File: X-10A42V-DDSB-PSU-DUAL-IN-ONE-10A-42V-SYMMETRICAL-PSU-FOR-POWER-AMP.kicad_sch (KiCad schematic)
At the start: 61 parts, among them K101 SLA-24VDC-SL-A, SW101 JWMW21RA1A, T101 15A

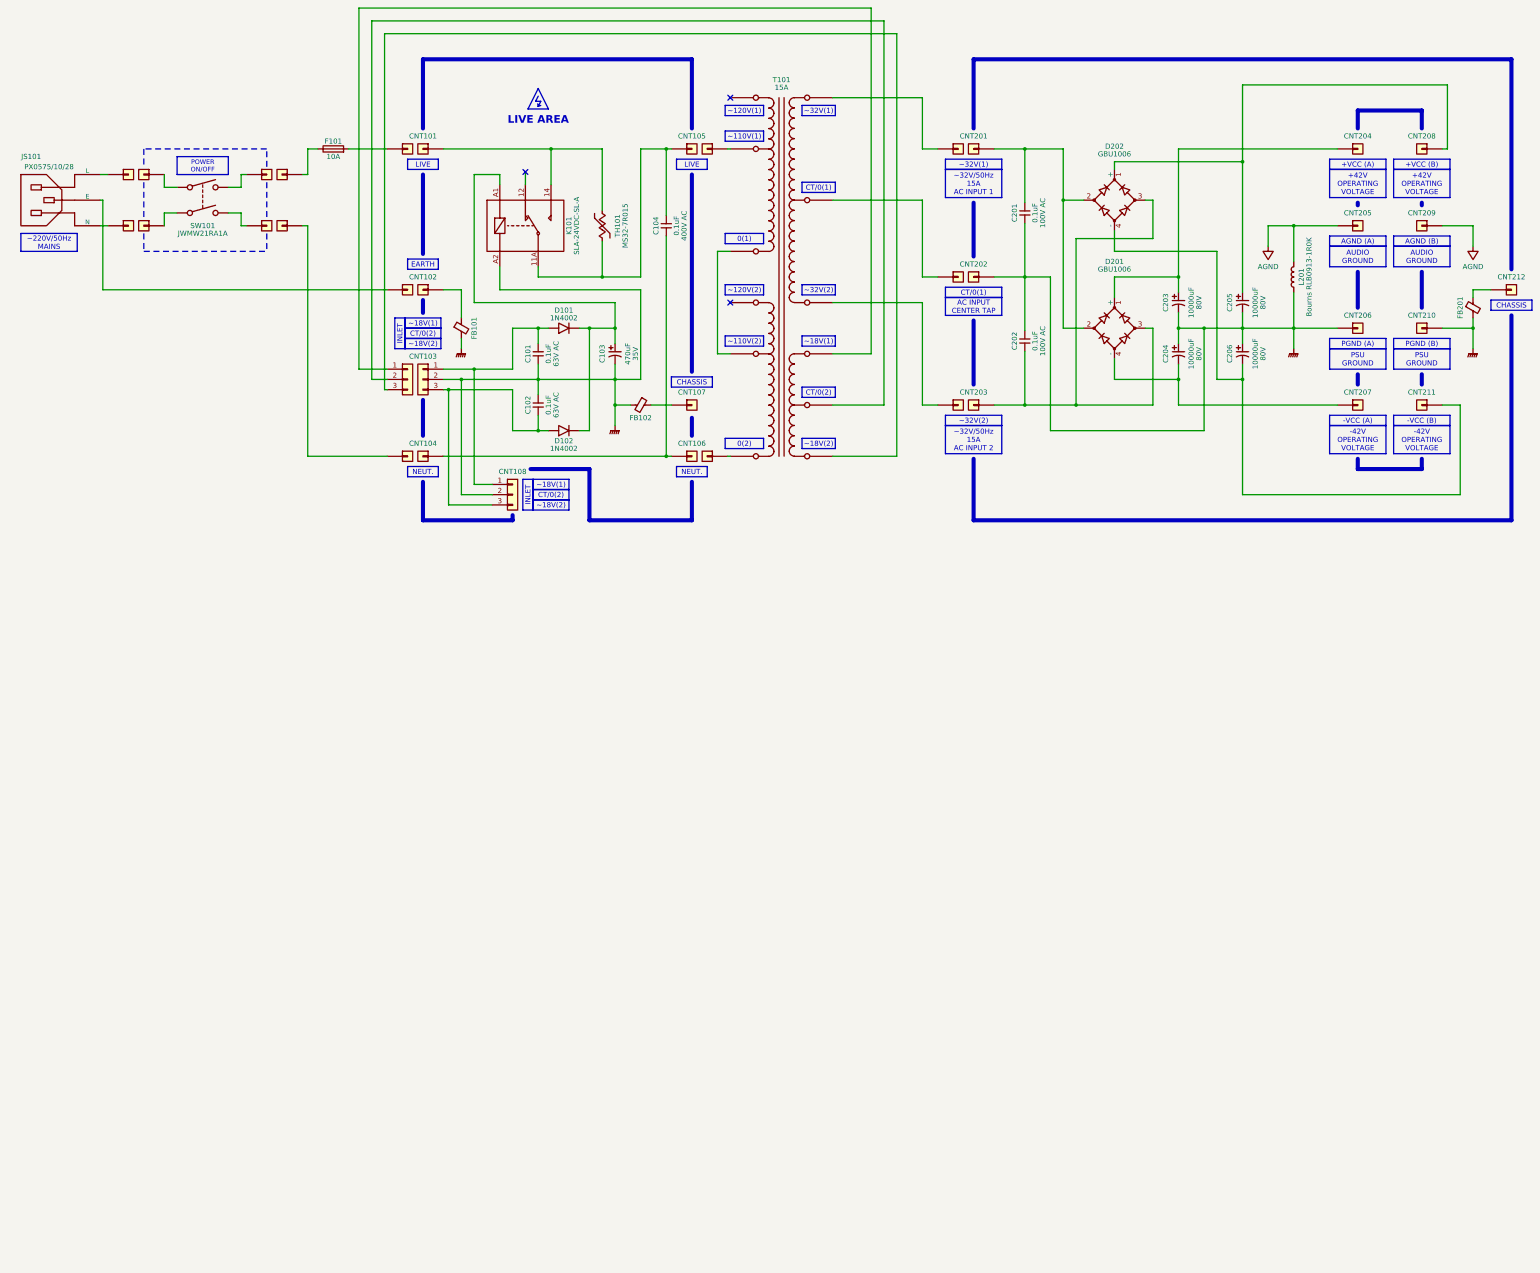
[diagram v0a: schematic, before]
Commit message: Update
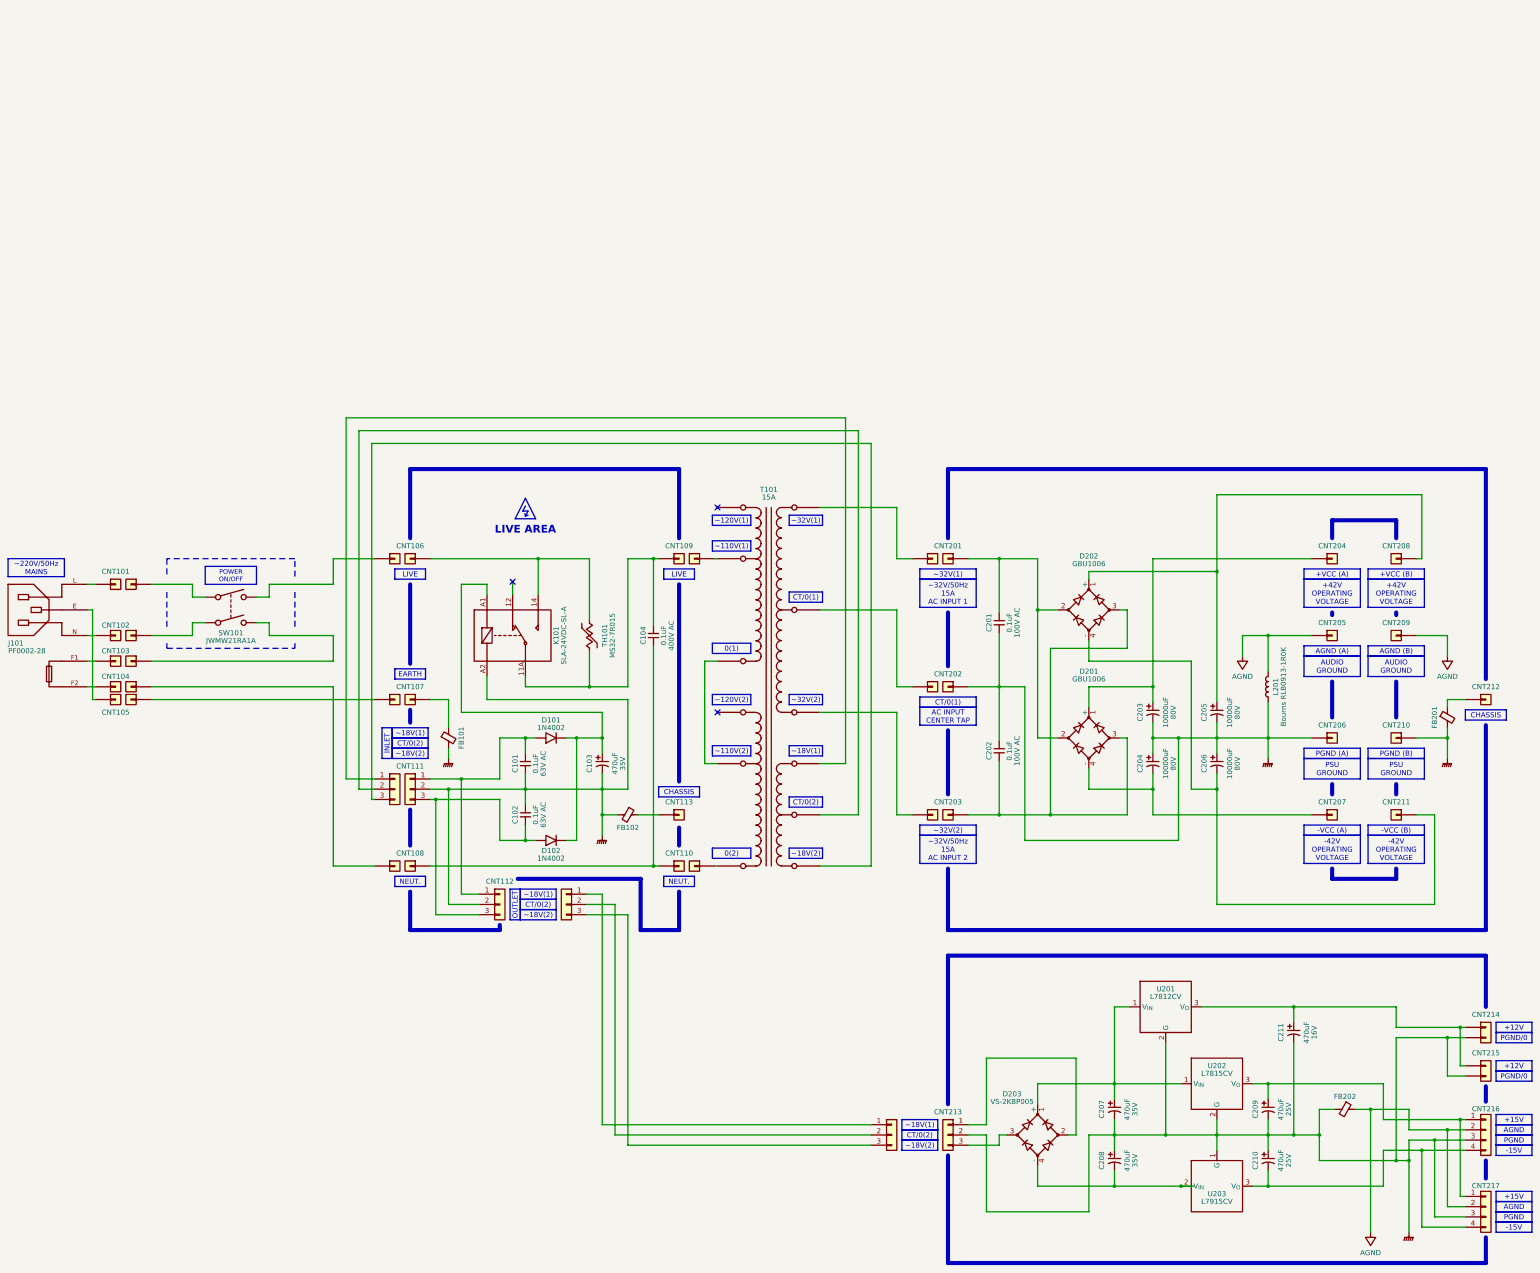
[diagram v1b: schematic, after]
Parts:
- removed CNTX101, CNTX102, CNTX105, CNTX106, CNTX107, CNTX108: 2376582-2, CUSTOM-FOOTPRINTS:PCB_TAB_250_FASTON_TPBR, symbol Connector_Generic:Conn_01x01
- removed F101: 10A, symbol Device:Fuse
- removed JS101: PX0575/10/28, CUSTOM-FOOTPRINTS:J_12.7mm, symbol CUSTOM-SYMBOLS:AC_POWER_ENTRY_SOCKET
- added C207, C208, C209, C210, C211: 470uF, CUSTOM-FOOTPRINTS:CP_Radial_D10.0mm_P5.00mm, symbol CUSTOM-SYMBOLS:C_Polarized_Small_US
- added CNT101, CNT102, CNT103, CNT104, CNT105: 2376582-2, CUSTOM-FOOTPRINTS:PCB_TAB_250_FASTON_TPBR, symbol Connector_Generic:Conn_01x01
- added CNT213: 22-27-2031, CUSTOM-FOOTPRINTS:Molex_KK-254_AE-6410-03A_1x03_P2.54mm_Vertical, symbol Connector_Generic:Conn_01x03
- added CNT214, CNT215: 22-27-2021, CUSTOM-FOOTPRINTS:Molex_KK-254_AE-6410-02A_1x02_P2.54mm_Vertical, symbol Connector_Generic:Conn_01x02
- added CNT216, CNT217: 22-27-2041, CUSTOM-FOOTPRINTS:Molex_KK-254_AE-6410-04A_1x04_P2.54mm_Vertical, symbol Connector_Generic:Conn_01x04
- added CNTX204, CNTX205: 10-11-2034, symbol Connector_Generic:Conn_01x03
- added CNTX206, CNTX207, CNTX208: 1-160304-8, CUSTOM-FOOTPRINTS:PCB_TAB_250_FASTON_TPBR, symbol Connector_Generic:Conn_01x01
- added D203: VS-2KBP005, CUSTOM-FOOTPRINTS:Diode_Bridge_Vishay_KBPM, symbol CUSTOM-SYMBOLS:D_Bridge_+AA-
- added FB202: Ferrite Bead, Ferrite_THT:LairdTech_28C0236-0JW-10, symbol Device:FerriteBead_Small
- added J101: PF0002-28, CUSTOM-FOOTPRINTS:BULGIN-IEC-Connector-PF0002-28, symbol CUSTOM-SYMBOLS:AC_POWER_ENTRY_SOCKET_WITH_FUSE
- added U201: L7812CV, CUSTOM-FOOTPRINTS:TO-220-3_Vertical_Heatsink-SK-104_38.1mm, symbol CUSTOM-SYMBOLS:78XX
- added U202: L7815CV, CUSTOM-FOOTPRINTS:TO-220-3_Vertical_Heatsink-SK-104_38.1mm, symbol CUSTOM-SYMBOLS:78XX
- added U203: L7915CV, CUSTOM-FOOTPRINTS:TO-220-3_Vertical_Heatsink-SK-104_38.1mm, symbol CUSTOM-SYMBOLS:79XX
- CNTX103, CNTX104, CNTX109, CNTX110, CNTX112, CNTX113, CNTX114, CNTX201, CNTX202, CNTX203: value 2376582-2 -> 1-160304-8; MFR Number 2376582-2 -> 1-160304-8
- CNTX111: value 22-27-2031 -> 10-11-2034; footprint CUSTOM-FOOTPRINTS:Molex_KK-254_AE-6410-04A_1x04_P2.54mm_Vertical -> (none); MFR Number 22-27-2031 -> 10-11-2034
- renumbered CNT101 to CNT106, CNT102 to CNT107, CNT104 to CNT108, CNT105 to CNT109, CNT106 to CNT110, CNT103 to CNT111, CNT108 to CNT112, CNT107 to CNT113
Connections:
- net at CNTX109.1 (Pin_1): now also SW101.2
- net at CNTX112.1 (Pin_1): now also CNTX207.1 (Pin_1)
- net at SW101.4: now also CNTX208.1 (Pin_1)
- net at CNTX110.1 (Pin_1): now also CNTX206.1 (Pin_1)
- new net: C209.1, CNT216.1 (Pin_1), CNT217.1 (Pin_1), U202.3 (V_{O})
- new net: C210.2, CNT216.4 (Pin_4), CNT217.4 (Pin_4), U203.3 (V_{O})
- new net: C211.1, CNT214.1 (Pin_1), CNT215.1 (Pin_1), U201.3 (V_{O})
- new net: CNT104.1 (Pin_1), J101.F2
- new net: C208.2, D203.4 (-), U203.2 (V_{IN})
- new net: C207.1, D203.1 (+), U201.1 (V_{IN}), U202.1 (V_{IN})
- new net: CNT213.1 (Pin_1), D203.2
- new net: CNT213.3 (Pin_3), D203.3
- new net: CNTX204.1 (Pin_1), CNTX205.1 (Pin_1)
- new net: CNTX204.2 (Pin_2), CNTX205.2 (Pin_2)
- new net: CNTX204.3 (Pin_3), CNTX205.3 (Pin_3)
- new net: CNT105.1 (Pin_1), J101.E
- new net: CNT102.1 (Pin_1), J101.N
- new net: CNT103.1 (Pin_1), J101.F1
- new net: CNT101.1 (Pin_1), J101.L
- new net AGND2: CNT216.2 (Pin_2), CNT217.2 (Pin_2), FB202.1
- new net PGND2: C207.2, C208.1, C209.2, C210.1, C211.2, CNT213.2 (Pin_2), CNT214.2 (Pin_2), CNT215.2 (Pin_2), CNT216.3 (Pin_3), CNT217.3 (Pin_3), FB202.2, U201.2 (G), U202.2 (G), U203.1 (G)
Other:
- moved on the sheet: C101, C102, C103, C104, C201, C202, C203, C204, C205, C206, CNT106, CNT107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
